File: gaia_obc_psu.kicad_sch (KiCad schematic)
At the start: 69 parts, among them IC1 MAX17048G+T10, Q2 FS8205A, SW8 SW_Slide_DPDT, U10 TPS22917DBV, U11 AP2112K-3.3, U12 DW01A, U13 AP2112K-3.0, U14 LGS4056HDB, U4 INA3221, U5 INA3221, U6 TPS22917DBV, U7 TPS22917DBV, U8 TPS22917DBV, U9 TPS22917DBV

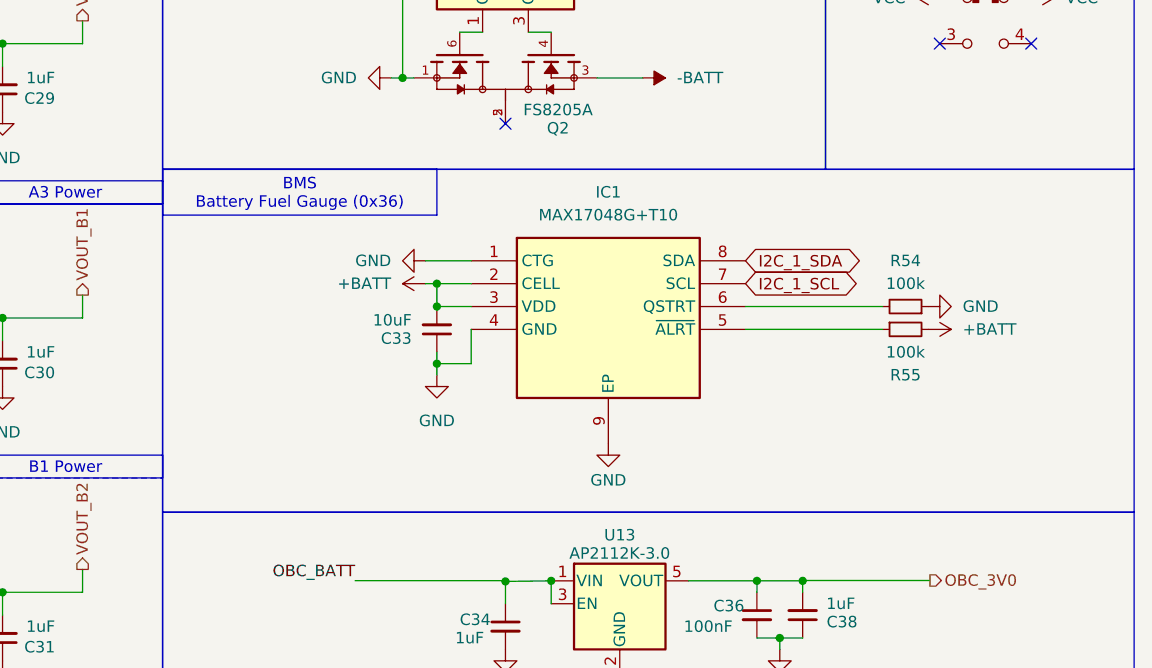
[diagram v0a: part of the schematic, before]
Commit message: v1.2
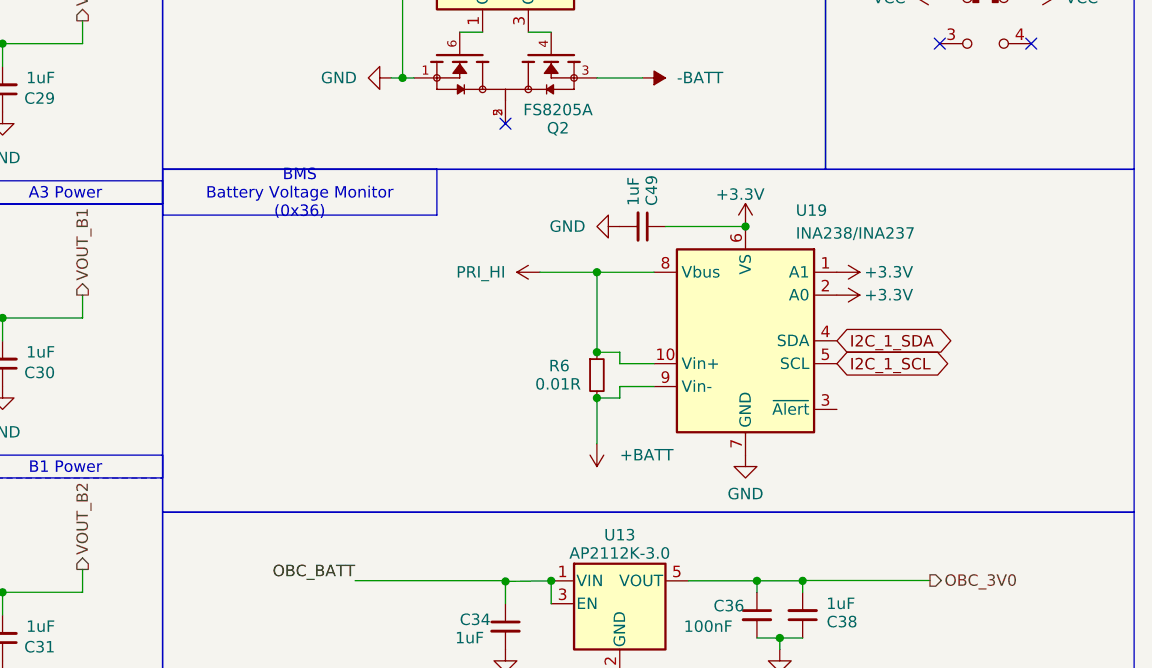
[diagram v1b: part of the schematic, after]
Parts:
- removed C33: 10uF, Capacitor_SMD:C_0603_1608Metric, symbol Device:C_Small
- removed IC1: MAX17048G+T10, gaia_obc-footprints:SON50P200X200X80-9N-D, symbol gaia_obc-symbols:MAX17048G+T10
- removed R54, R55: 100k, Resistor_SMD:R_0603_1608Metric, symbol Device:R_Small
- added C49: 1uF, Capacitor_SMD:C_0603_1608Metric, symbol Device:C_Small
- added R6: 0.01R, Resistor_SMD:R_2512_6332Metric, symbol Device:R_Small
- added U19: INA238/INA237, Package_SO:VSSOP-10_3x3mm_P0.5mm, symbol Sensor_Energy:INA238
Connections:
- net +3.3V: now also C49.1, U19.1 (A1), U19.2 (A0), U19.6 (VS)
- net +BATT: now also R6.2, U19.9 (Vin-)
- net GND: now also C49.2, U19.7 (GND)
- net I2C_1_SCL: now also U19.5 (SCL)
- net I2C_1_SDA: now also U19.4 (SDA)
- new net PRI_HI: R6.1, U19.10 (Vin+), U19.8 (Vbus)
